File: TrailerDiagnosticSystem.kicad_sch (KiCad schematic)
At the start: 2 parts, among them J3 Conn_01x10, J4 Conn_01x10

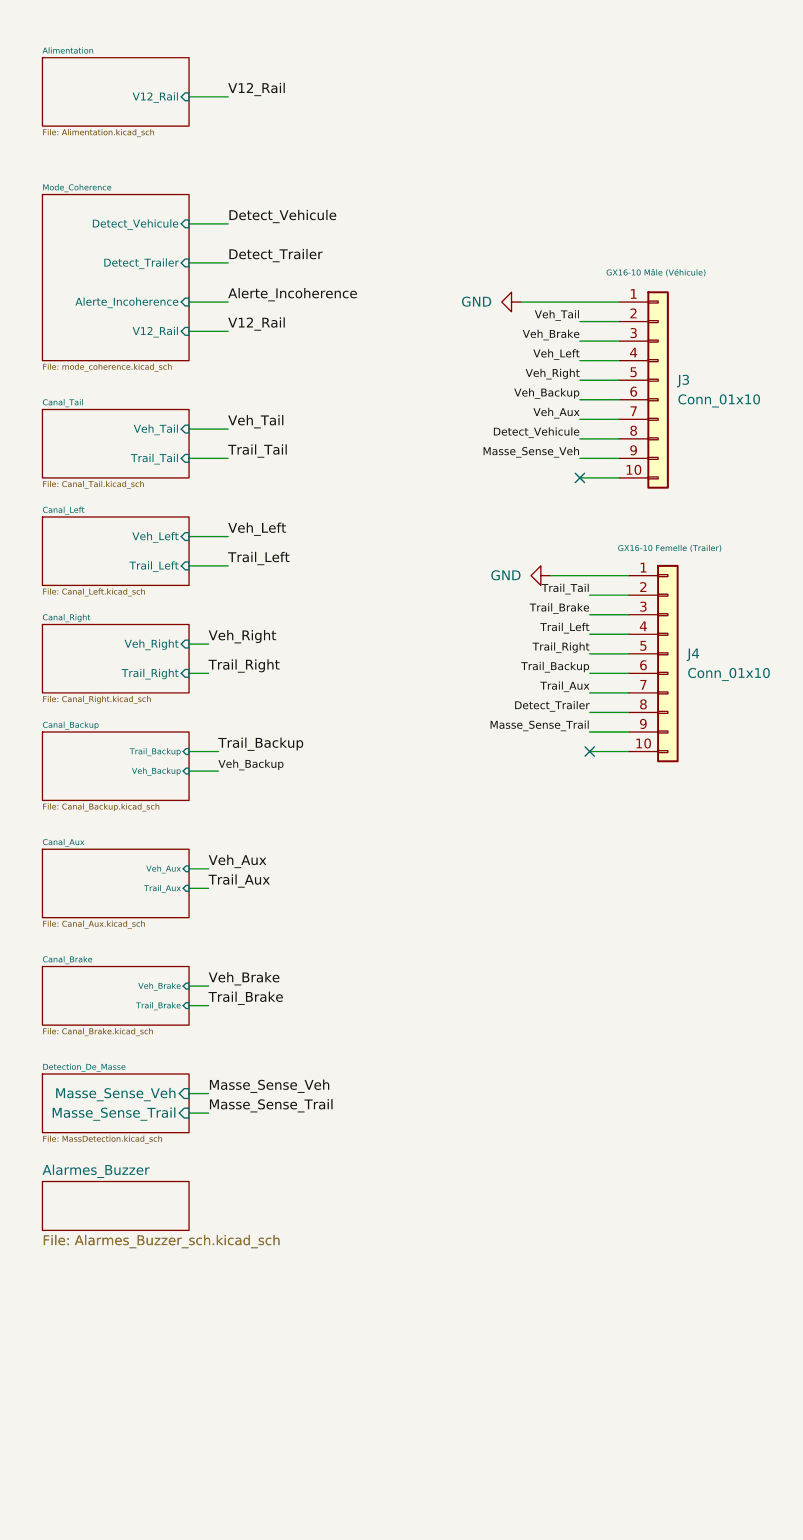
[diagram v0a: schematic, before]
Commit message: Add files via upload
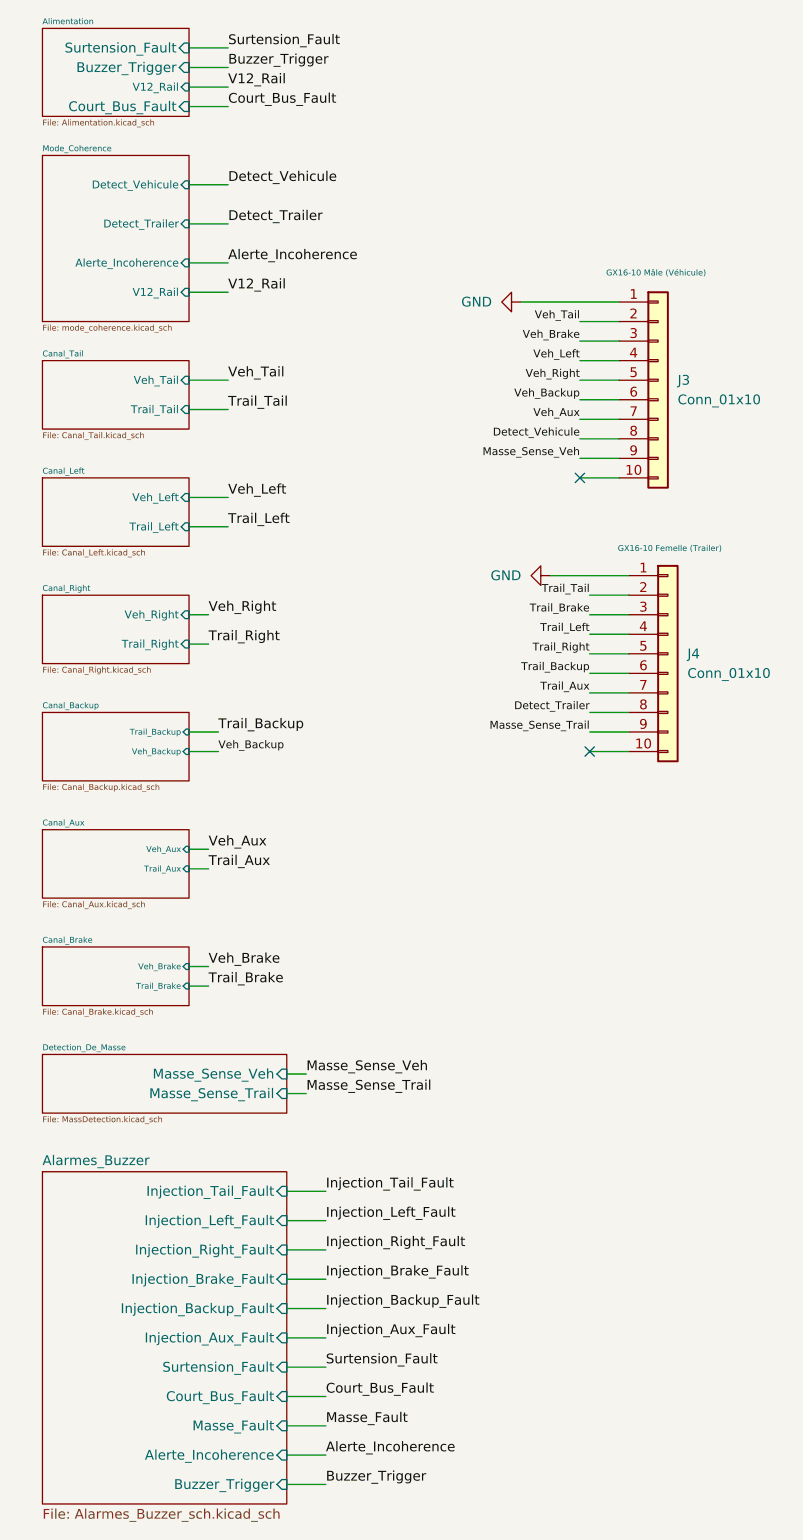
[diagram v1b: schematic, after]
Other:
- sheet Alarmes_Buzzer ports: added Alerte_Incoherence, Buzzer_Trigger, Court_Bus_Fault, Injection_Aux_Fault, Injection_Backup_Fault, Injection_Brake_Fault, Injection_Left_Fault, Injection_Right_Fault, Injection_Tail_Fault, Masse_Fault, Surtension_Fault; removed none
- sheet Alimentation ports: added Buzzer_Trigger, Court_Bus_Fault, Surtension_Fault; removed none

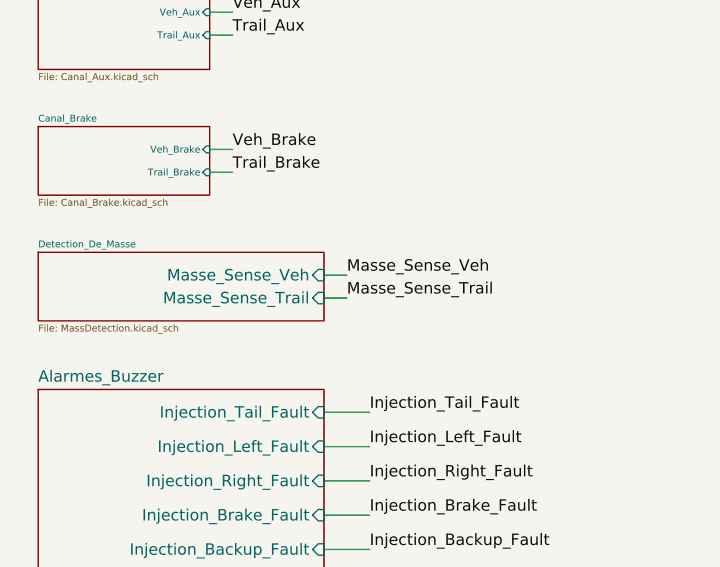
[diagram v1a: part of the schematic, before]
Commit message: Add files via upload
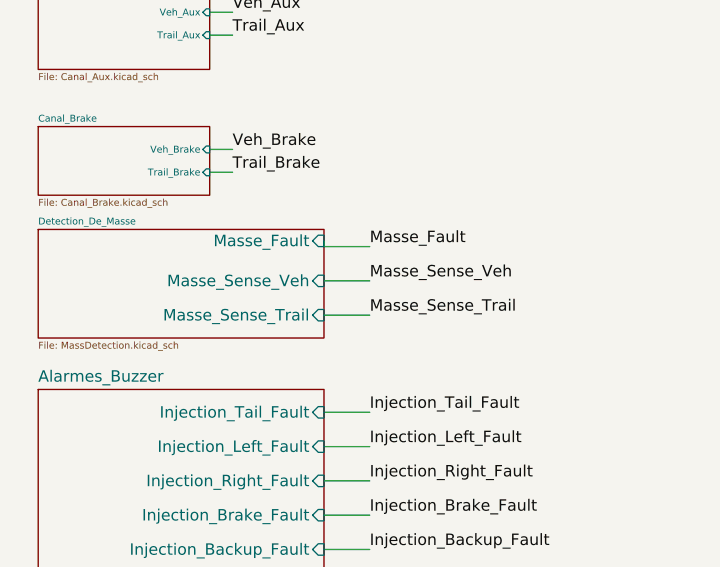
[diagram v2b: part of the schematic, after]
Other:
- sheet Detection_De_Masse ports: added Masse_Fault; removed none
